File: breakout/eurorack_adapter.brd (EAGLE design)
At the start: 13 x 14.1 mm, 5 parts

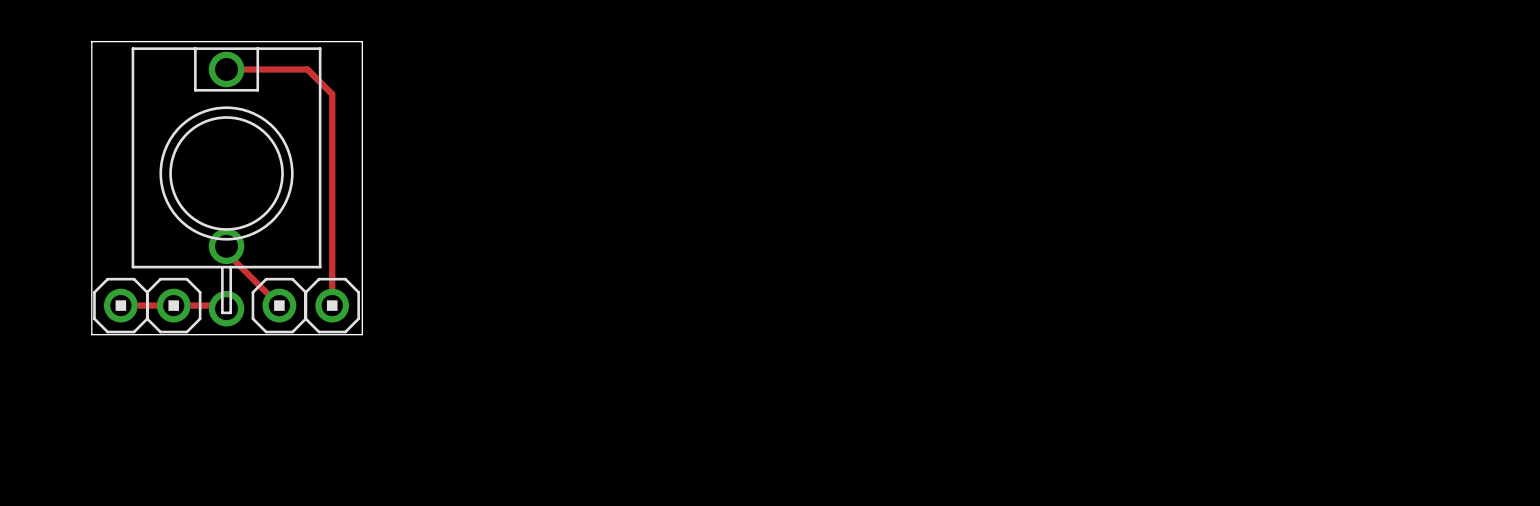
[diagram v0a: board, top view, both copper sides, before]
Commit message: Changes
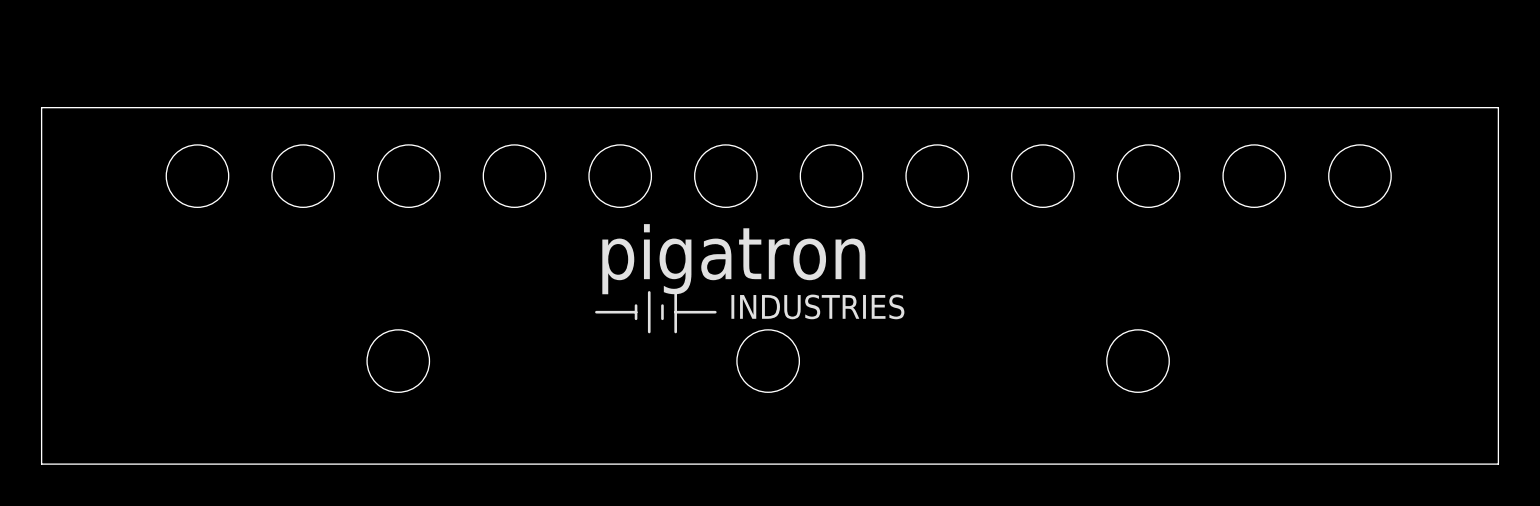
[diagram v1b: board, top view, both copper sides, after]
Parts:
- removed GND, GND1, NORM, SIG: HEADER/MALE/01, connectors:HEADER/MALE/01
- U$1: value WQP-PJ301M-12_JACK -> (none); device controls:WQP-PJ301M-12_JACK -> mechanical:PIGATRON-LOGO
- moved U$1 27.1 mm to (35.6, 8.89)
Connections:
- removed net N$1: SIG.1, U$1.P$1
- removed net N$2: NORM.1, U$1.P$2
- removed net N$6: GND.1, GND1.1, U$1.P$3
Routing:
- net N$1: track 15.7 -> 0.00 mm
- net N$6: track 5.14 -> 0.00 mm
- net N$2: track 3.90 -> 0.00 mm
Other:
- board size 13 x 14.1 mm -> 70 x 17.1 mm
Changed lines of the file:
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@@
 <settings>
 <setting alwaysvectorfont="no"/>
+<setting keepoldvectorfont="yes"/>
 <setting verticaltext="up"/>
 </settings>
-<grid distance="50" unitdist="mil" unit="mil" style="lines" multiple="1" display="no" altdistance="10" altunitdist="mil" altunit="mil"/>
+<grid distance="50" unitdist="mil" unit="mil" style="lines" multiple="1" display="no" altdistance="5" altunitdist="mil" altunit="mil"/>
 <layers>
 <layer number="1" name="Top" color="4" fill="1" visible="yes" active="yes"/>
@@
 <layer number="43" name="vRestrict" color="2" fill="10" visible="yes" active="yes"/>
 <layer number="44" name="Drills" color="7" fill="1" visible="no" active="yes"/>
-<layer number="45" name="Holes" color="7" fill="1" visible="no" active="yes"/>
+<layer number="45" name="Holes" color="7" fill="1" visible="yes" active="yes"/>
 <layer number="46" name="Milling" color="3" fill="1" visible="no" active="yes"/>
 <layer number="47" name="Measures" color="7" fill="1" visible="no" active="yes"/>
@@
 <board>
 <plain>
-<wire x1="2.413" y1="6.223" x2="15.418" y2="6.223" width="0" layer="20"/>
-<wire x1="15.418" y1="6.223" x2="15.418" y2="20.31" width="0" layer="20"/>
-<wire x1="15.418" y1="20.31" x2="2.413" y2="20.31" width="0" layer="20"/>
-<wire x1="2.413" y1="20.31" x2="2.413" y2="6.223" width="0" layer="20"/>
+<wire x1="0" y1="0" x2="70.028" y2="0" width="0" layer="20"/>
+<wire x1="70.028" y1="0" x2="70.028" y2="17.135" width="0" layer="20"/>
+<wire x1="70.028" y1="17.135" x2="0" y2="17.135" width="0" layer="20"/>
+<wire x1="0" y1="17.135" x2="0" y2="0" width="0" layer="20"/>
+<dimension x1="0" y1="0" x2="0" y2="149.86" x3="-7.62" y3="74.93" textsize="1.778" layer="48"/>
+<dimension x1="0" y1="10.668" x2="0" y2="139.192" x3="-3.81" y3="74.93" textsize="1.778" layer="48"/>
+<dimension x1="0" y1="149.86" x2="0" y2="139.065" x3="6.35" y3="144.4625" textsize="1.778" layer="48"/>
+<hole x="7.493" y="13.843" drill="2.99999375"/>
+<hole x="12.573" y="13.843" drill="2.99999375"/>
+<hole x="17.653" y="13.843" drill="2.99999375"/>
+<hole x="22.733" y="13.843" drill="2.99999375"/>
+<hole x="27.813" y="13.843" drill="2.99999375"/>
+<hole x="32.893" y="13.843" drill="2.99999375"/>
+<hole x="37.973" y="13.843" drill="2.99999375"/>
+<hole x="43.053" y="13.843" drill="2.99999375"/>
+<hole x="48.133" y="13.843" drill="2.99999375"/>
+<hole x="53.213" y="13.843" drill="2.99999375"/>
+<hole x="58.293" y="13.843" drill="2.99999375"/>
+<hole x="63.373" y="13.843" drill="2.99999375"/>
+<dimension x1="0" y1="0" x2="70.028" y2="0" x3="35.014" y3="-3.81" textsize="1.778" layer="48"/>
+<hole x="34.925" y="4.953" drill="2.99999375"/>
+<hole x="17.145" y="4.953" drill="2.99999375"/>
+<hole x="52.705" y="4.953" drill="2.99999375"/>
 </plain>
 <attributes>
@@
 </autorouter>
 <elements>
-<element name="GND" library="connectors" package="HEADER/MALE/01" value="HEADER/MALE/01" x="3.81" y="7.62" smashed="yes" rot="R90">
-<attribute name="NAME" x="4.572" y="9.525" size="1.016" layer="26" ratio="10" rot="MR90"/>
-</element>
-<element name="NORM" library="connectors" package="HEADER/MALE/01" value="HEADER/MALE/01" x="11.43" y="7.62" smashed="yes" rot="R90">
-<attribute name="NAME" x="10.922" y="9.525" size="1.016" layer="26" ratio="10" rot="MR90"/>
-</element>
-<element name="SIG" library="connectors" package="HEADER/MALE/01" value="HEADER/MALE/01" x="13.97" y="7.62" smashed="yes" rot="R90">
-<attribute name="NAME" x="13.462" y="9.525" size="1.016" layer="26" ratio="10" rot="MR90"/>
-</element>
-<element name="U$1" library="controls" package="WQP-PJ301M-12_JACK" value="WQP-PJ301M-12_JACK" x="8.89" y="13.97" smashed="yes"/>
-<element name="GND1" library="connectors" package="HEADER/MALE/01" value="HEADER/MALE/01" x="6.35" y="7.62" smashed="yes"/>
+<element name="U$1" library="mechanical" package="PIGATRON-LOGO" value="" x="35.56" y="8.89" smashed="yes"/>
 </elements>
 <signals>
-<signal name="N$1">
-<contactref element="U$1" pad="P$1"/>
-<contactref element="SIG" pad="1"/>
-<wire x1="13.97" y1="7.62" x2="13.97" y2="17.78" width="0.3048" layer="1"/>
-<wire x1="13.97" y1="17.78" x2="12.78" y2="18.97" width="0.3048" layer="1"/>
-<wire x1="12.78" y1="18.97" x2="8.89" y2="18.97" width="0.3048" layer="1"/>
-</signal>
-<signal name="N$2">
-<contactref element="U$1" pad="P$2"/>
-<contactref element="NORM" pad="1"/>
-<wire x1="11.43" y1="7.62" x2="8.89" y2="10.16" width="0.3048" layer="1"/>
-<wire x1="8.89" y1="10.16" x2="8.89" y2="10.47" width="0.3048" layer="1"/>
-</signal>
-<signal name="N$6">
-<contactref element="U$1" pad="P$3"/>
-<contactref element="GND" pad="1"/>
-<contactref element="GND1" pad="1"/>
-<wire x1="3.81" y1="7.62" x2="6.35" y2="7.62" width="0.3048" layer="1"/>
-<wire x1="6.35" y1="7.62" x2="8.74" y2="7.62" width="0.3048" layer="1"/>
-<wire x1="8.74" y1="7.62" x2="8.89" y2="7.47" width="0.3048" layer="1"/>
-</signal>
 </signals>
 <mfgpreviewcolors>
